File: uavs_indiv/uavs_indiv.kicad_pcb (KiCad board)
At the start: 2 copper layers, 46.5 x 159.5 mm, 16 parts, among them J4 Conn_01x04_Pin, J5 Conn_01x04_Pin, J6 Conn_01x04_Pin, U1 LM2576HVS-5, U3 LM2576HVS-5

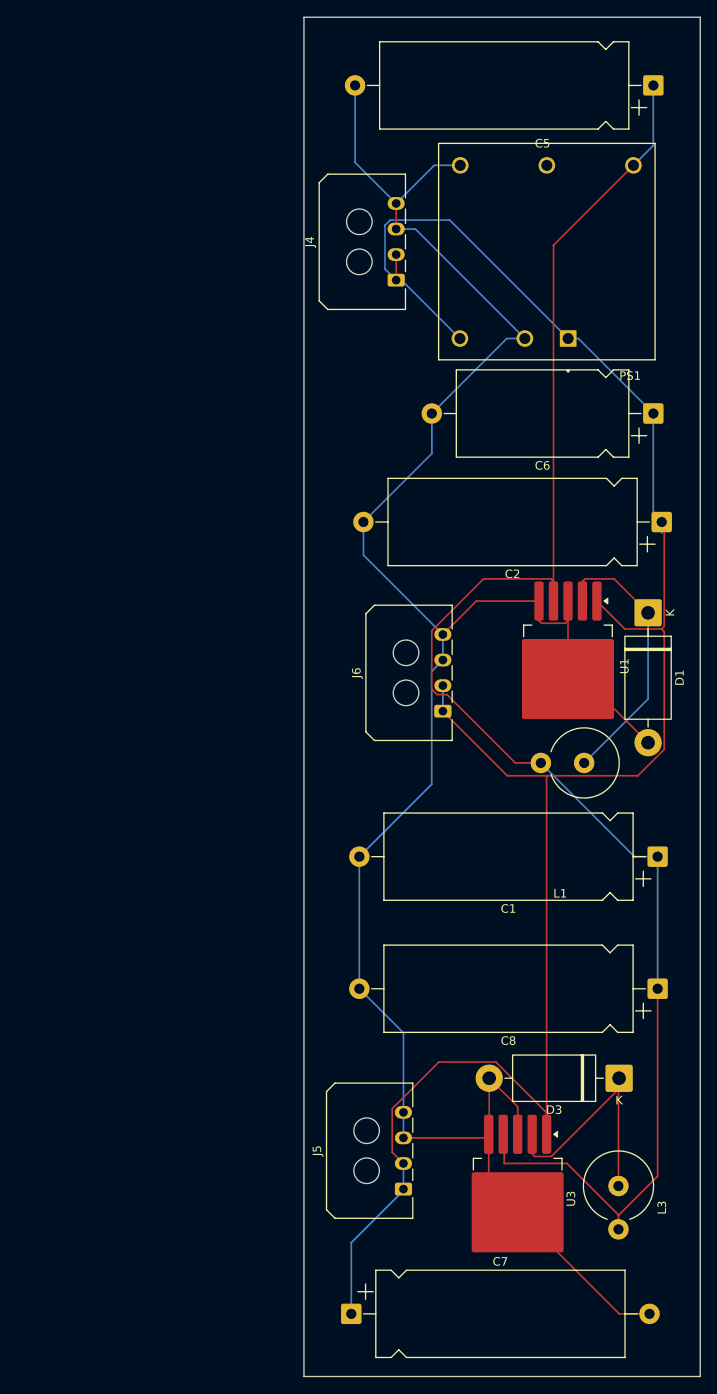
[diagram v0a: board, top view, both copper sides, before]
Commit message: wtf did i just see
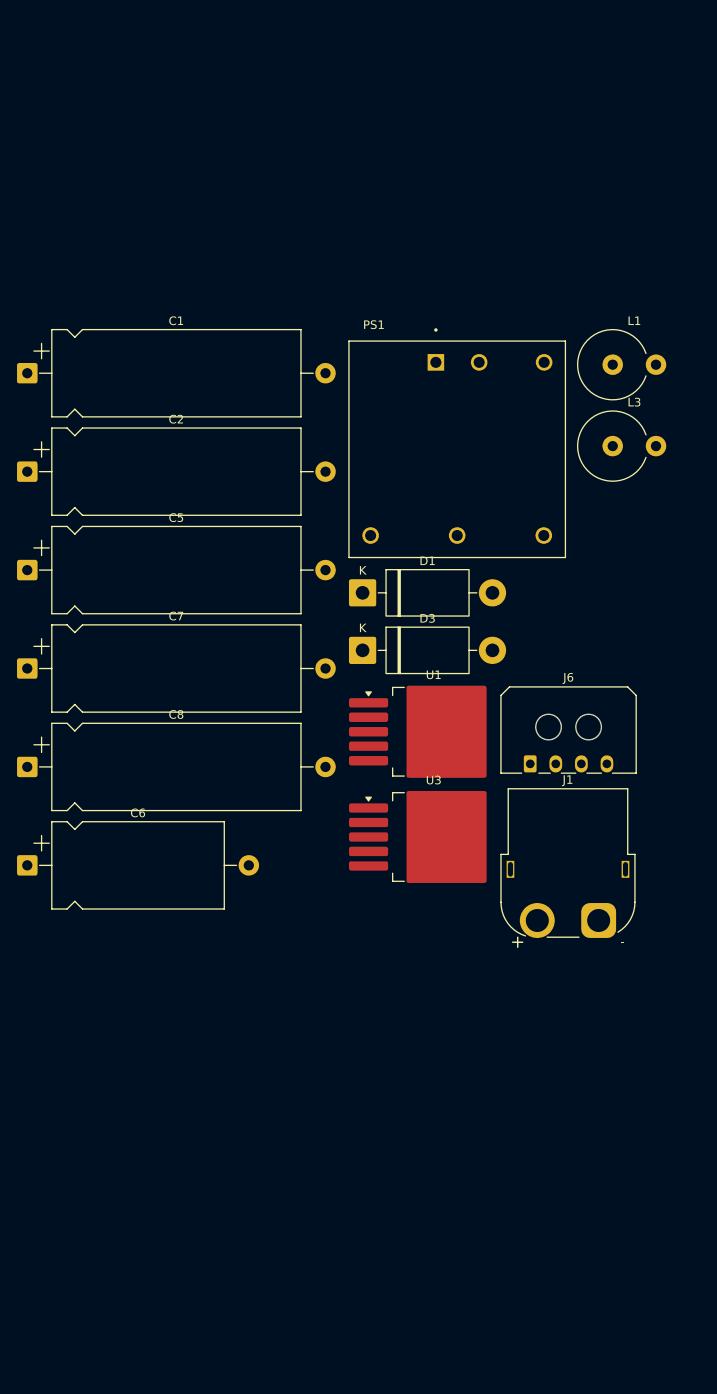
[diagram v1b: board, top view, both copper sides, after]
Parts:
- removed J4, J5: Conn_01x04_Pin, customdcdc:Molex_Micro-Fit_3.0_43650-0400_1x04_P3.00mm_Horizontal
- added J1: Conn_01x02_Socket, Connector_AMASS:AMASS_XT60PW-F_1x02_P7.20mm_Horizontal, F.Cu at (140.1, 126.5)
- moved C1 93.2 mm to (73.0, 62.3), turned to 0 degrees
- moved C5 92.9 mm to (73.0, 85.4), turned to 0 degrees
- moved C6 90.6 mm to (73.0, 120.0), turned to 0 degrees
- moved L3 86.8 mm to (141.7, 70.8), turned to 0 degrees
- moved C7 84.7 mm to (73.0, 96.9)
- moved C8 78.4 mm to (73.0, 108.5), turned to 0 degrees
- moved C2 74.7 mm to (73.0, 73.8), turned to 0 degrees
- moved D3 58.5 mm to (112.4, 94.8), turned to 0 degrees
- moved L1 46.9 mm to (141.7, 61.3), turned to 0 degrees
- moved U3 43.7 mm to (120.7, 116.7), turned to 0 degrees
- moved D1 33.6 mm to (112.4, 88.0), turned to 0 degrees
- moved PS1 25.5 mm to (123.5, 71.2), turned to 0 degrees
- moved U1 17.5 mm to (120.7, 104.3), turned to 0 degrees
- moved J6 12.0 mm to (132.1, 108.1), turned to 0 degrees
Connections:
- J6 pad 1: /Vin -> +5V
- J6 pad 2: /Vin -> +5V
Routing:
- net GND: track 260.3 -> 0.00 mm
- net /Vin: track 241.3 -> 0.00 mm
- net +5V: track 191.2 -> 0.00 mm
- net Net-(D1-K): track 34.2 -> 0.00 mm
- net Net-(D3-K): track 29.8 -> 0.00 mm
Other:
- board outline removed
